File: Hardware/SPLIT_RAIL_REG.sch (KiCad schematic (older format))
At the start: 21 parts, among them Q1 PMOS, U1 TPS65130

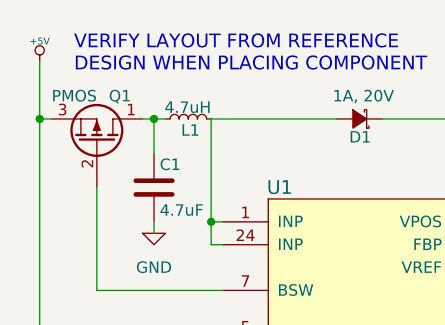
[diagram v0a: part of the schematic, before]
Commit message: (Digital) board fixes
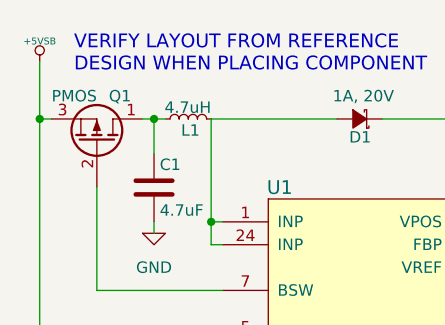
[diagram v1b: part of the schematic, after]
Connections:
- net +5V renamed +5VSB
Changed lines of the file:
@@
 Sourced 976K\nfor R1
 $Comp
-L +5V #PWR013
-U 1 1 5862836D
+L +5VSB #PWR013
+U 1 1 586D4235
 P 4050 2300
 F 0 "#PWR013" H 4050 2390 20  0001 C CNN
-F 1 "+5V" H 4050 2390 30  0000 C CNN
+F 1 "+5VSB" H 4050 2390 30  0000 C CNN
 F 2 "" H 4050 2300 60  0000 C CNN
 F 3 "" H 4050 2300 60  0000 C CNN
